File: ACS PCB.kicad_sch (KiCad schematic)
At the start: 4 parts, among them J5 Conn_01x02

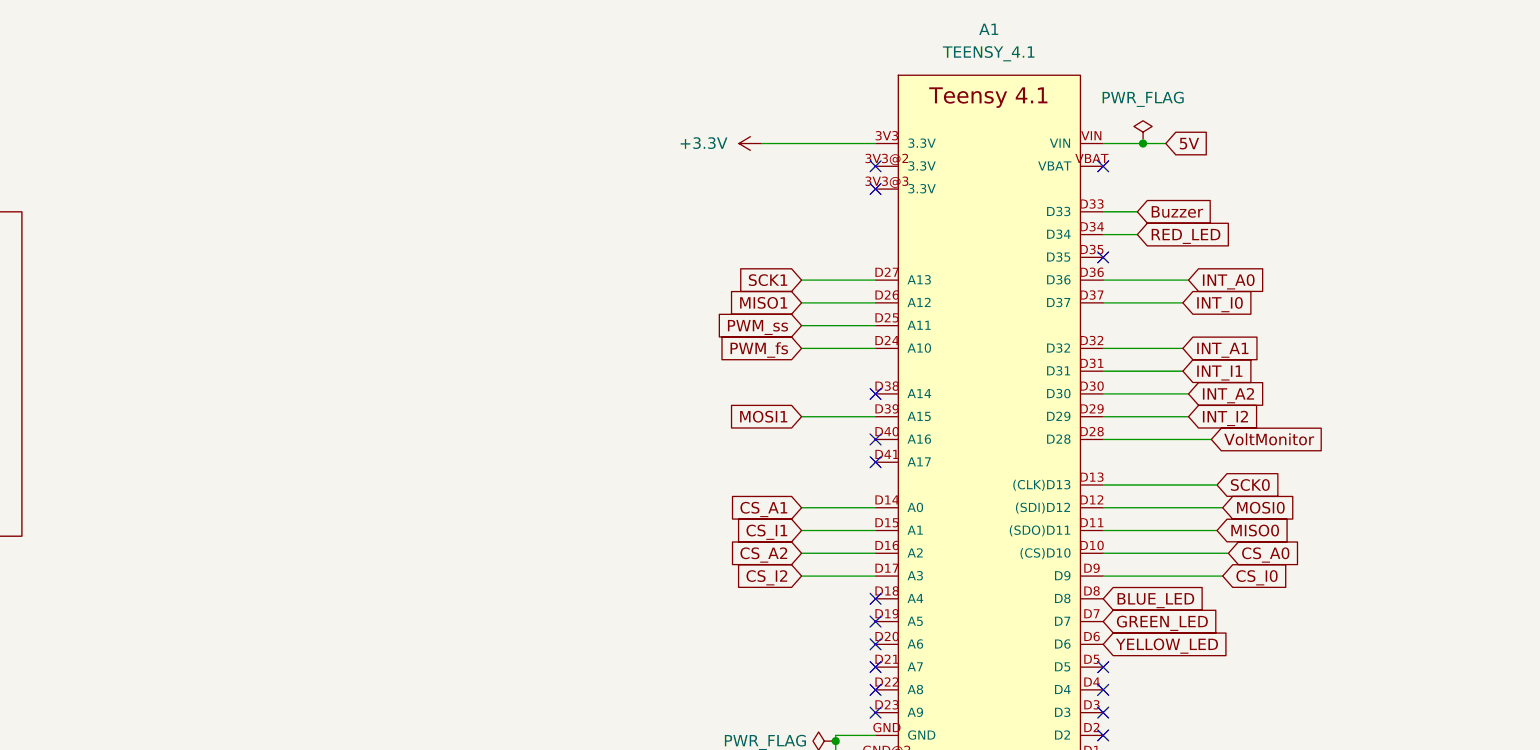
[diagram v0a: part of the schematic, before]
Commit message: miso-mosi-fix
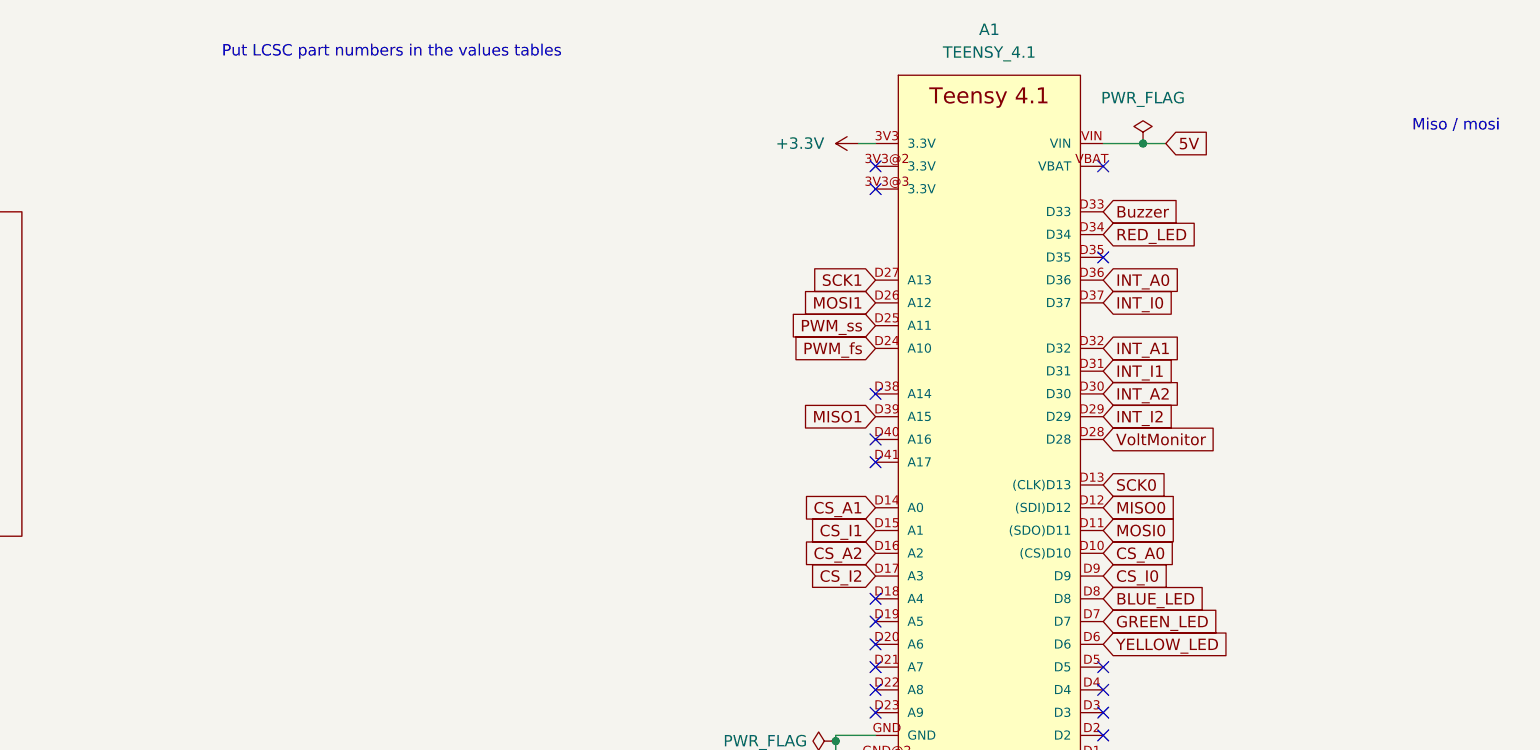
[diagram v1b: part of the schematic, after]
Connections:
- net MISO0: now also A1.D12 ((SDI)D12); no longer A1.D11 ((SDO)D11)
- net MISO1: now also A1.D39 (A15); no longer A1.D26 (A12)
- net MOSI0: now also A1.D11 ((SDO)D11); no longer A1.D12 ((SDI)D12)
- net MOSI1: now also A1.D26 (A12); no longer A1.D39 (A15)
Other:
- note added: "Miso / mosi"
- note added: "Put LCSC part numbers in the values tables"

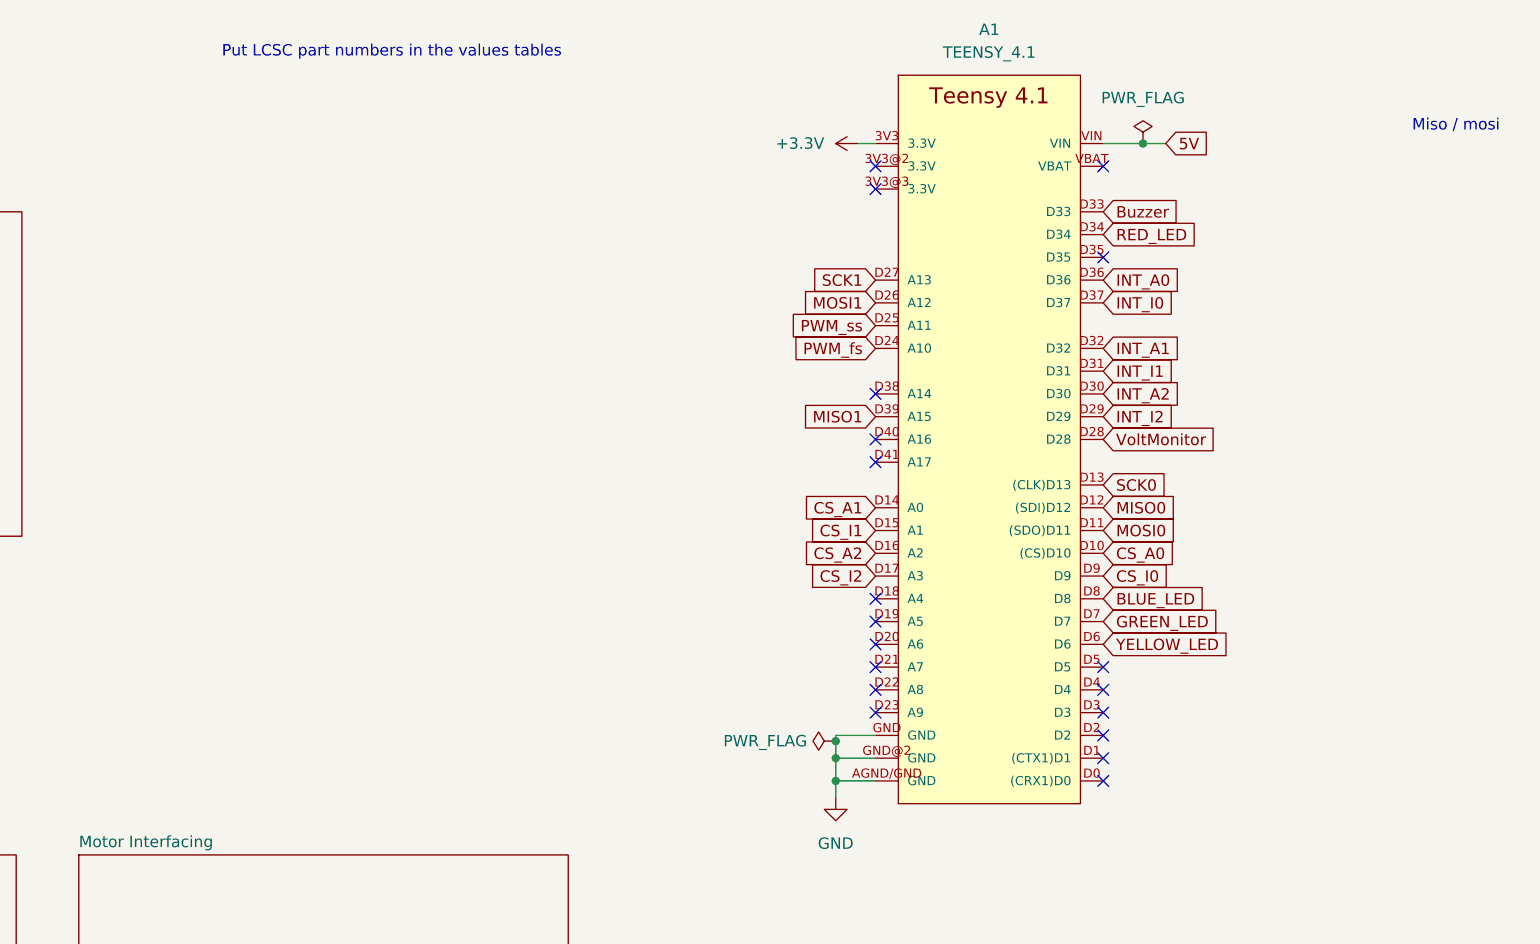
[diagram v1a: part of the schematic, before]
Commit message: created PCB and layout
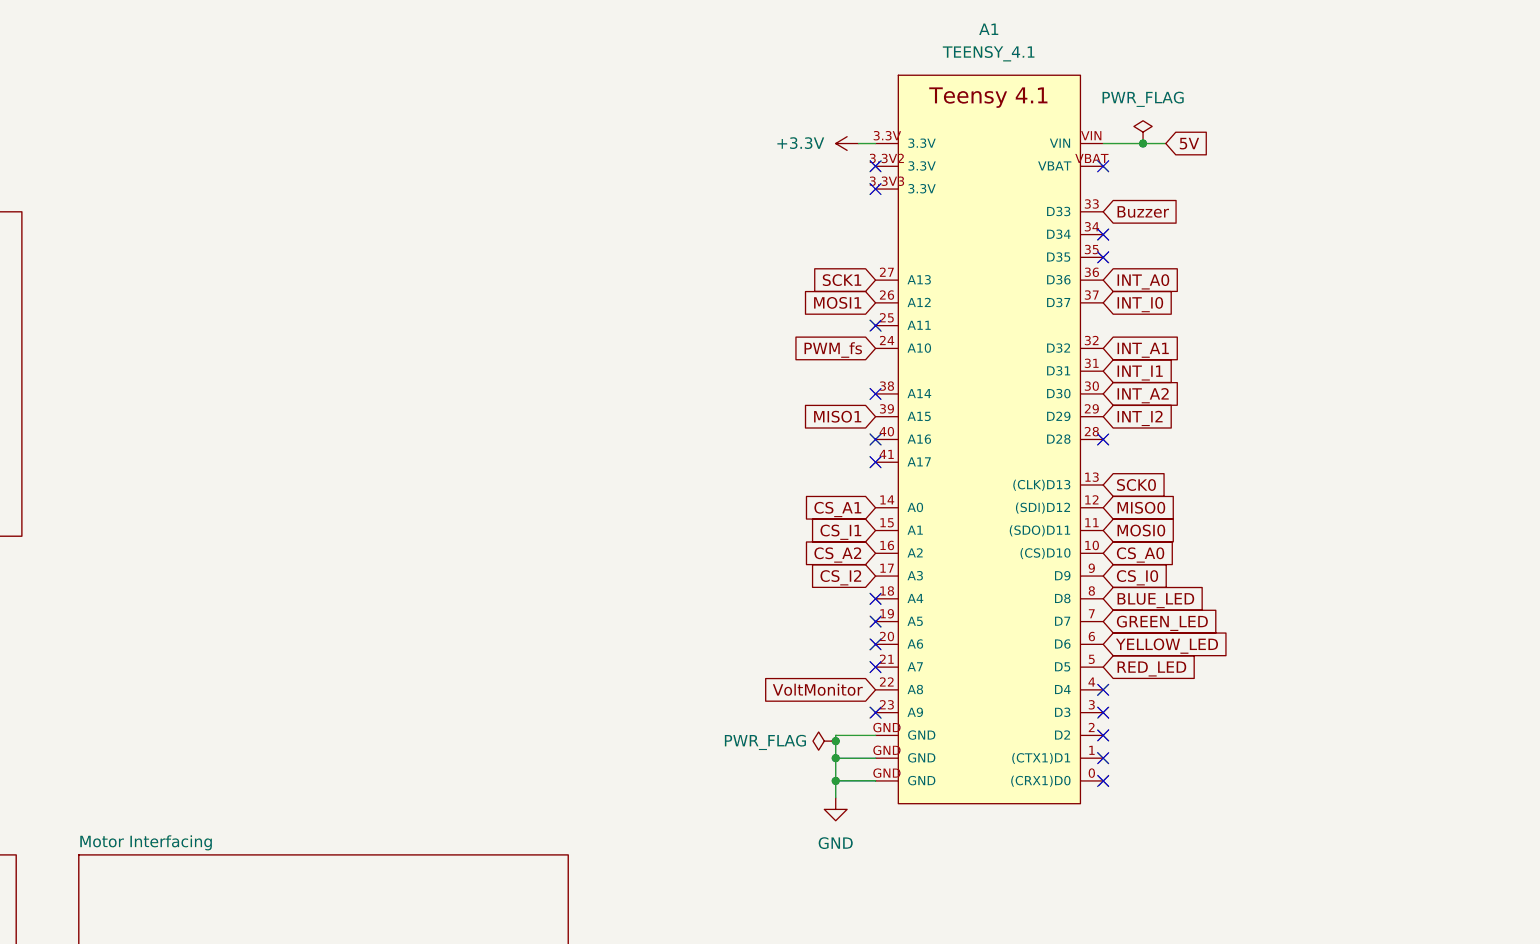
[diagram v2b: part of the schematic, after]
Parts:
- A1: footprint Teensy:Teensy41 -> Teensy 4.1:Teensy41
- D5: footprint (none) -> Diode_SMD:D_SMC
- F1: footprint (none) -> Fuse:Fuse_1206_3216Metric
- J5: footprint (none) -> Connector_AMASS:AMASS_XT60-F_1x02_P7.20mm_Vertical
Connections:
- net +3.3V: now also A1.3.3V; no longer A1.3V3 (3.3V)
- net BLUE_LED: now also A1.8 (D8); no longer A1.D8
- net Buzzer: now also A1.33 (D33); no longer A1.D33
- net CS_A0: now also A1.10 ((CS)D10); no longer A1.D10 ((CS)D10)
- net CS_A1: now also A1.14 (A0); no longer A1.D14 (A0)
- net CS_A2: now also A1.16 (A2); no longer A1.D16 (A2)
- net CS_I0: now also A1.9 (D9); no longer A1.D9
- net CS_I1: now also A1.15 (A1); no longer A1.D15 (A1)
- net CS_I2: now also A1.17 (A3); no longer A1.D17 (A3)
- net GND: no longer A1.AGND/GND (GND), A1.GND@2 (GND)
- net GREEN_LED: now also A1.7 (D7); no longer A1.D7
- net INT_A0: now also A1.36 (D36); no longer A1.D36
- net INT_A1: now also A1.32 (D32); no longer A1.D32
- net INT_A2: now also A1.30 (D30); no longer A1.D30
- net INT_I0: now also A1.37 (D37); no longer A1.D37
- net INT_I1: now also A1.31 (D31); no longer A1.D31
- net INT_I2: now also A1.29 (D29); no longer A1.D29
- net MISO0: now also A1.12 ((SDI)D12); no longer A1.D12 ((SDI)D12)
- net MISO1: now also A1.39 (A15); no longer A1.D39 (A15)
- net MOSI0: now also A1.11 ((SDO)D11); no longer A1.D11 ((SDO)D11)
- net MOSI1: now also A1.26 (A12); no longer A1.D26 (A12)
- net PWM_fs: now also A1.24 (A10); no longer A1.D24 (A10)
- net RED_LED: now also A1.5 (D5); no longer A1.D34
- net SCK0: now also A1.13 ((CLK)D13); no longer A1.D13 ((CLK)D13)
- net SCK1: now also A1.27 (A13); no longer A1.D27 (A13)
- net VoltMonitor: now also A1.22 (A8); no longer A1.D28
- net YELLOW_LED: now also A1.6 (D6); no longer A1.D6
- removed net PWM_ss: A1.D25 (A11)
- no-connect marks 19 -> 20
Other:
- note removed: "Miso / mosi"
- note removed: "Put LCSC part numbers in the values tables"
- moved on the sheet: A1
